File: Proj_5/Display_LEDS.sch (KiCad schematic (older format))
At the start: 6 parts, among them J1 DSUB-9, J2 DSUB-9, U27 max235cpg

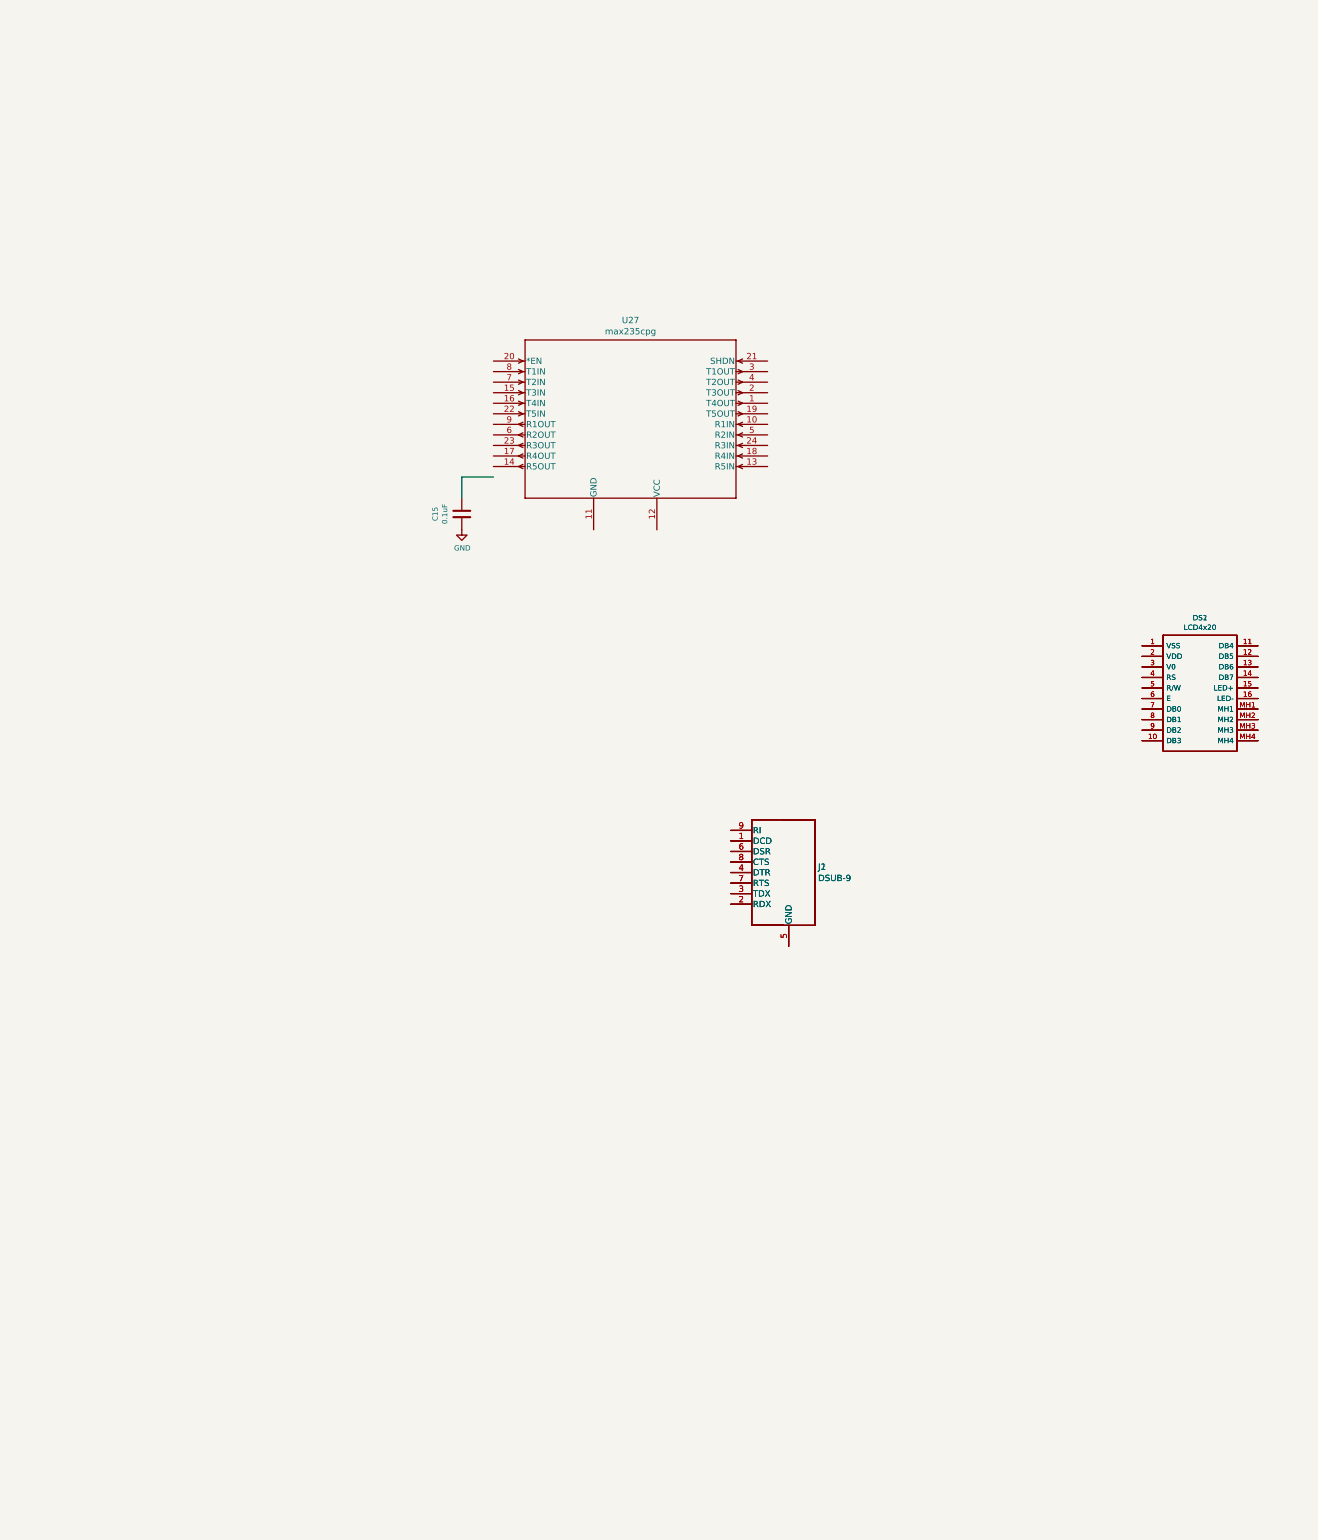
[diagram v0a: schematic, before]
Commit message: LCD boop
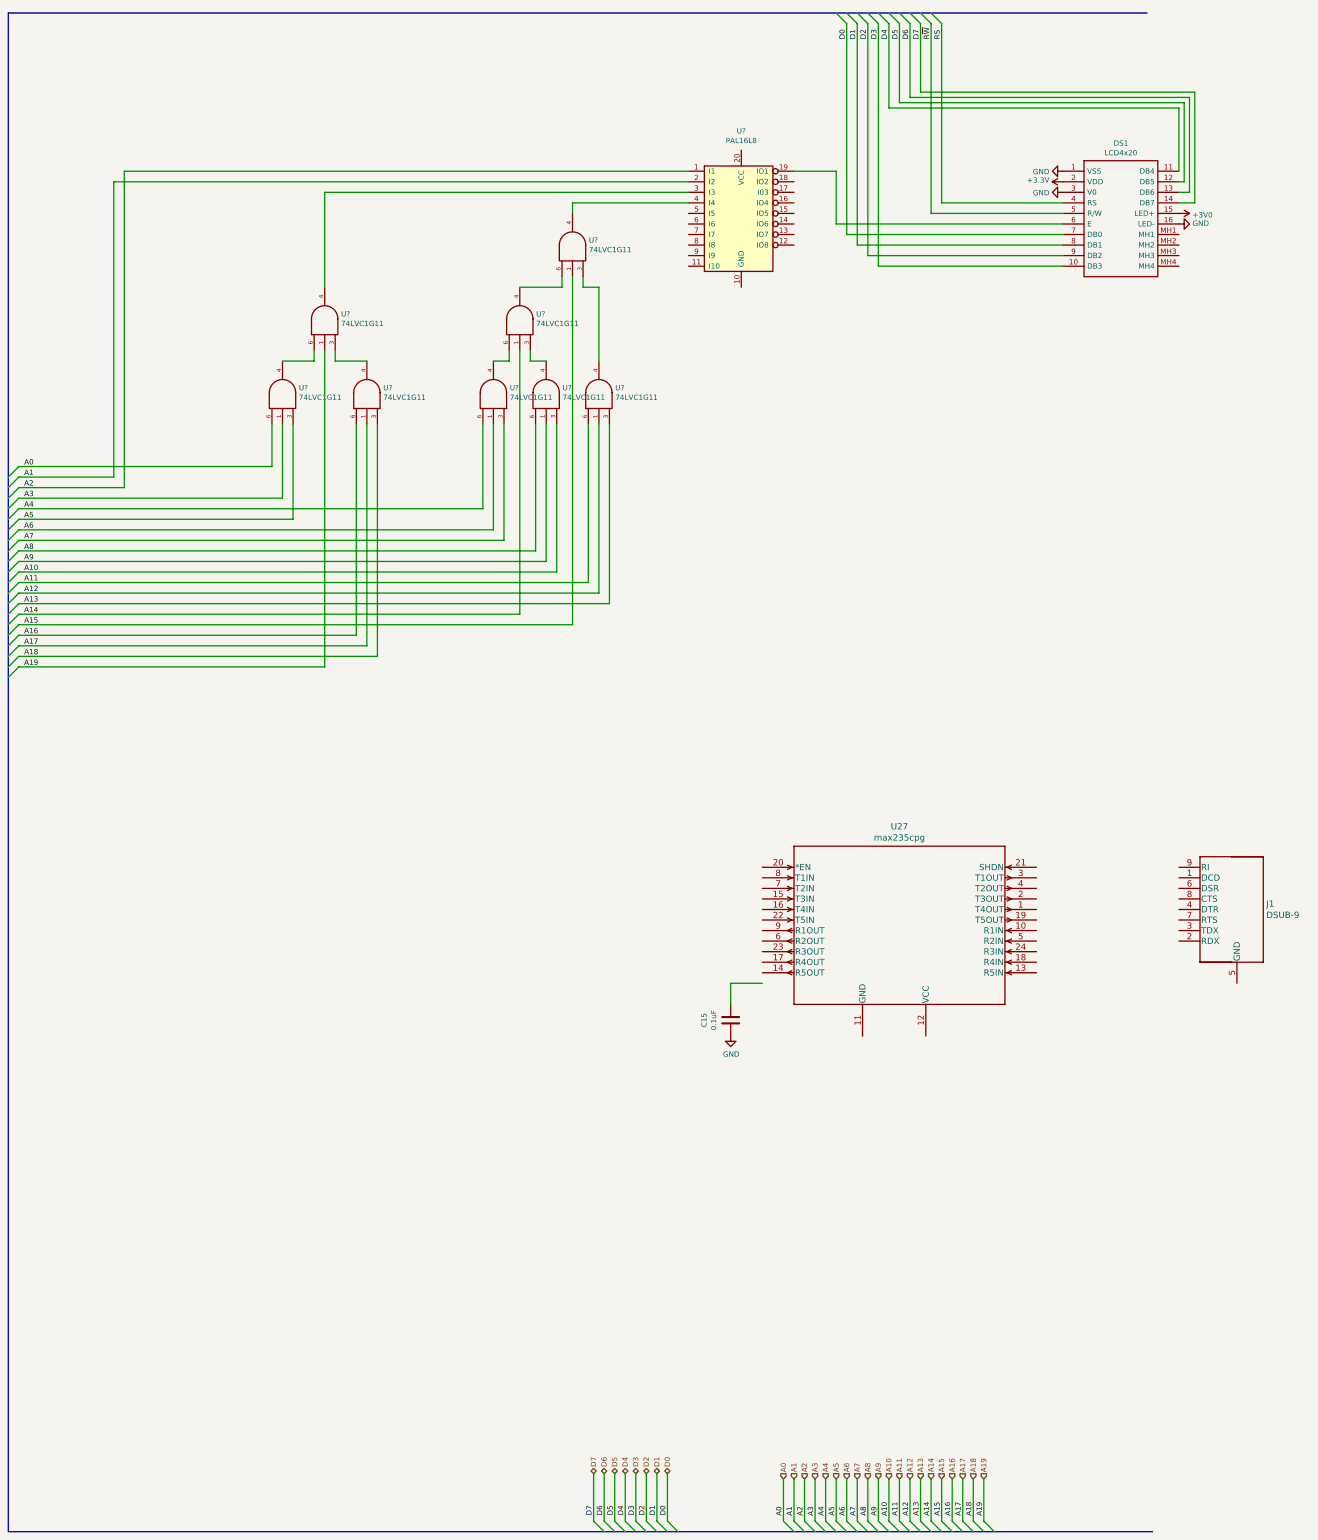
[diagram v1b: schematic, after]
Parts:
- removed DS2: LCD4x20, LCD4x20, symbol LCD4x20:LCD4x20
- removed J2: DSUB-9, DSUB-9, symbol DSUB-9:DSUB-9
- added U?: PAL16L8, symbol Logic_Programmable:PAL16L8
- added U? (x8): 74LVC1G11, symbol 74xGxx:74LVC1G11
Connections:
- net labels added: +3.3V, +3V0, A0, A1, A10, A11, A12, A13, A14, A15, A16, A17, A18, A19, A2, A3, A4, A5, A6, A7, A8, A9, D0, D1, D2, D3, D4, D5, D6, D7, RS, R~W
- wire segments 2 -> 119
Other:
- moved on the sheet: C15, DS1, J1, U27
